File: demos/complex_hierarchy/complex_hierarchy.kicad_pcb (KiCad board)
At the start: 2 copper layers, 72 parts, among them P1 CONN_2, P2 CONN_2, P3 CONN_2, P4 CONN_2, P5 CONN_2, P6 CONN_2, Q1 MPAS92, Q2 MPAS42, Q3 MPAS92, Q4 MPAS42, Q5 MPAS92, Q6 MPAS42, Q7 MPAS92, Q8 MPAS42, U1 ICL7660, U2 78L05, U3 LM358N, U4 LM358N

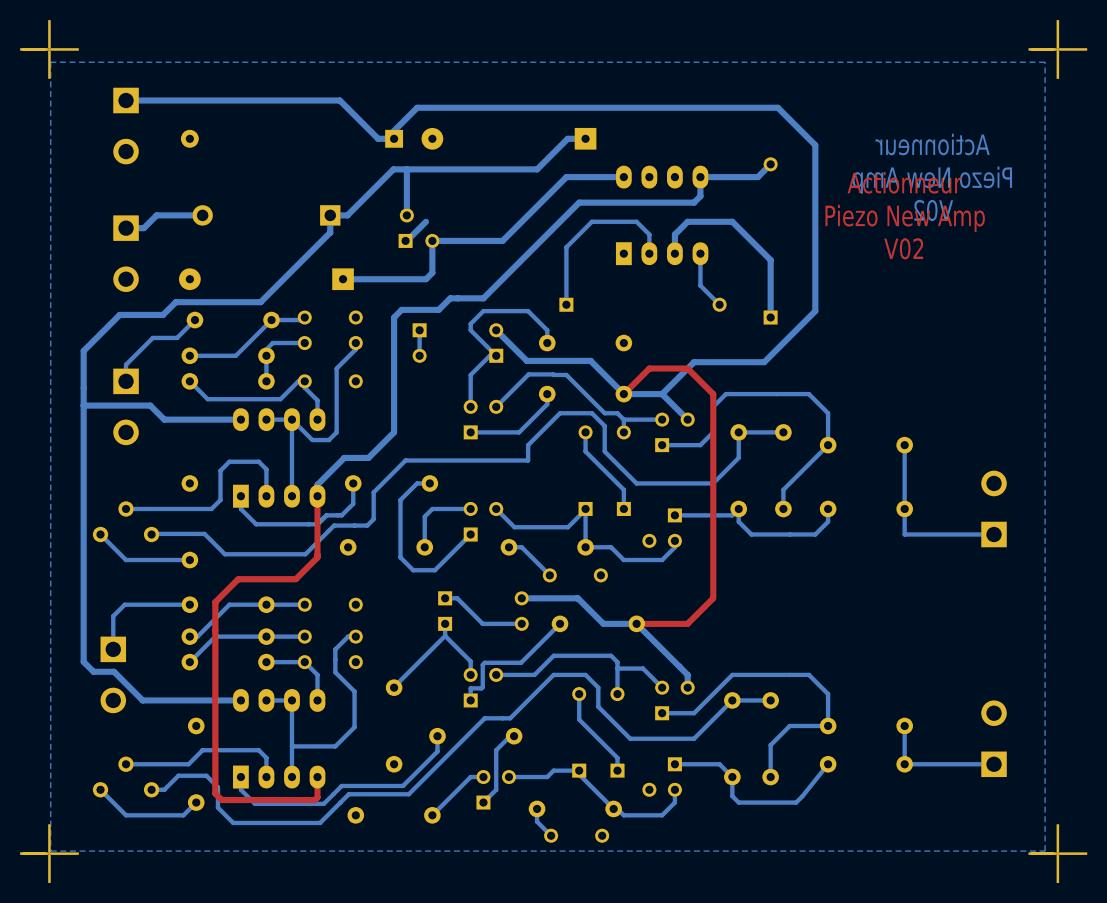
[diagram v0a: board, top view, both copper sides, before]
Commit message: Imported Upstream version 4.0.0~rc1
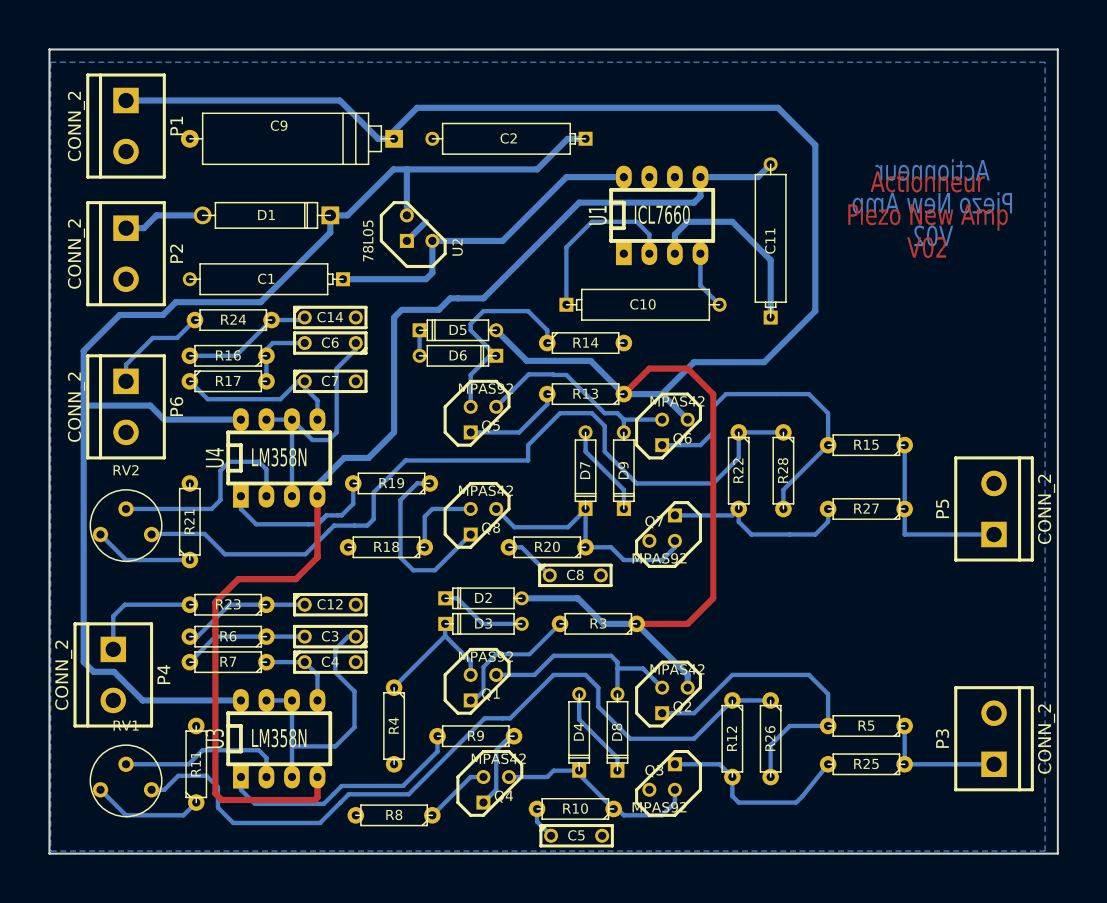
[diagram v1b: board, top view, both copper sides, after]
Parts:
- removed MIRE (x4): *, MIRE
- C1, C10, C11, C2: footprint CP6 -> discret:CP6
- C12, C14, C3, C5, C6, C8: footprint C2 -> discret:C2
- C4, C7: value 4,7nF -> 4.7nF; footprint C2 -> discret:C2
- C9: footprint CP8 -> discret:CP8
- D1: footprint D5 -> discret:D5
- D2, D3, D4, D5, D6, D7, D8, D9: footprint D3 -> discret:D3
- P1, P2, P3, P4, P5, P6: footprint bornier2 -> connect:bornier2
- Q1, Q2, Q3, Q4, Q5, Q6, Q7, Q8: footprint TO92-CBE -> discret:TO92-CBE
- R10, R11, R12, R13, R14, R15, R16, R17, R18, R19, R20, R21, R22, R23, R24, R25, R26, R27, R28, R3, R4, R5, R6, R7, R8, R9: footprint R3-LARGE_PADS -> discret:R3-LARGE_PADS
- RV1, RV2: footprint RV2 -> discret:RV2
- U1, U3, U4: footprint DIP-8__300_ELL -> dip_sockets:DIP-8__300_ELL
- U2: footprint LM78LXX -> discret:LM78LXX
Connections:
- net /ampli_h1 renamed /ampli_ht_vertical/Vpil_0_3,3V
- net /ampli_h2 renamed /ampli_ht_horizontal/Vpil_0_3,3V
- net /ampli_h3 renamed /ampli_ht_vertical/PIEZO_OUT
- net /ampli_h4 renamed /ampli_ht_vertical/PIEZO_IN
- net /ampli_h5 renamed /ampli_ht_horizontal/PIEZO_OUT
- net /ampli_h6 renamed /ampli_ht_horizontal/PIEZO_IN
- net /ampli_h7 renamed /ampli_ht_vertical/S_OUT+
- net /ampli_h8 renamed /ampli_ht_horizontal/S_OUT+
- D1 pad 1: /12Vext -> +12V
- D1 pad 2: +12V -> /12Vext
- D2 pad 1: HT -> Net-(D2-Pad1)
- D2 pad 2: N-000012 -> HT
- D3 pad 1: N-000012 -> Net-(D3-Pad1)
- D3 pad 2: N-000019 -> Net-(D2-Pad1)
- D4 pad 1: N-000023 -> Net-(D4-Pad1)
- D4 pad 2: N-000025 -> Net-(D4-Pad2)
- D5 pad 1: HT -> Net-(D5-Pad1)
- D5 pad 2: N-000033 -> HT
- D6 pad 1: N-000033 -> Net-(D6-Pad1)
- D6 pad 2: N-000040 -> Net-(D5-Pad1)
- D7 pad 1: N-000044 -> Net-(D7-Pad1)
- D7 pad 2: N-000046 -> Net-(D7-Pad2)
- D8 pad 1: N-000026 -> Net-(D4-Pad2)
- D8 pad 2: N-000023 -> Net-(D8-Pad2)
- D9 pad 1: N-000047 -> Net-(D7-Pad2)
- D9 pad 2: N-000044 -> Net-(D9-Pad2)
- Q1 pad B: N-000019 -> Net-(D3-Pad1)
- Q1 pad C: N-000026 -> Net-(D8-Pad2)
- Q2 pad B: N-000026 -> Net-(D8-Pad2)
- Q3 pad B: N-000025 -> Net-(D4-Pad1)
- Q4 pad C: N-000025 -> Net-(D4-Pad1)
- Q5 pad B: N-000040 -> Net-(D6-Pad1)
- Q5 pad C: N-000047 -> Net-(D9-Pad2)
- Q6 pad B: N-000047 -> Net-(D9-Pad2)
- Q7 pad B: N-000046 -> Net-(D7-Pad1)
- Q8 pad C: N-000046 -> Net-(D7-Pad1)
- R10 pad 1: N-000025 -> Net-(D4-Pad1)
- R14 pad 1: N-000040 -> Net-(D6-Pad1)
- R20 pad 1: N-000046 -> Net-(D7-Pad1)
- R4 pad 1: N-000019 -> Net-(D3-Pad1)
- U1 pad 6: (no net) -> Net-(U1-Pad6)
- U1 pad 7: (no net) -> Net-(U1-Pad7)
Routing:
- net Net-(D7-Pad1): track 0.00 -> 24.9 mm
- net N-000046: track 24.9 -> 0.00 mm
- net Net-(D8-Pad2): track 0.00 -> 21.5 mm
- net N-000026: track 21.5 -> 0.00 mm
- net Net-(D9-Pad2): track 0.00 -> 21.0 mm
- net N-000047: track 21.0 -> 0.00 mm
- net Net-(D6-Pad1): track 0.00 -> 20.9 mm
- net N-000040: track 20.9 -> 0.00 mm
- net Net-(D4-Pad1): track 0.00 -> 20.6 mm
- net N-000025: track 20.6 -> 0.00 mm
- net Net-(D3-Pad1): track 0.00 -> 13.4 mm
- net N-000019: track 13.4 -> 0.00 mm
- net Net-(D7-Pad2): track 0.00 -> 9.20 mm
- net Net-(D4-Pad2): track 0.00 -> 9.20 mm
- net N-000044: track 9.20 -> 0.00 mm
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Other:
- board outline added: 100.3 x 80 mm
- net class Default: clearance 0.2794 -> 0.3; trace_width 0.4318 -> 0.4
- net class power: clearance 0.381 -> 0.3; trace_width 0.6096 -> 0.6
- rule trace_clearance: 0.2794 -> 0.3
